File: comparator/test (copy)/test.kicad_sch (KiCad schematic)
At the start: 11 parts, among them Q4 NPN, Q5 NPN

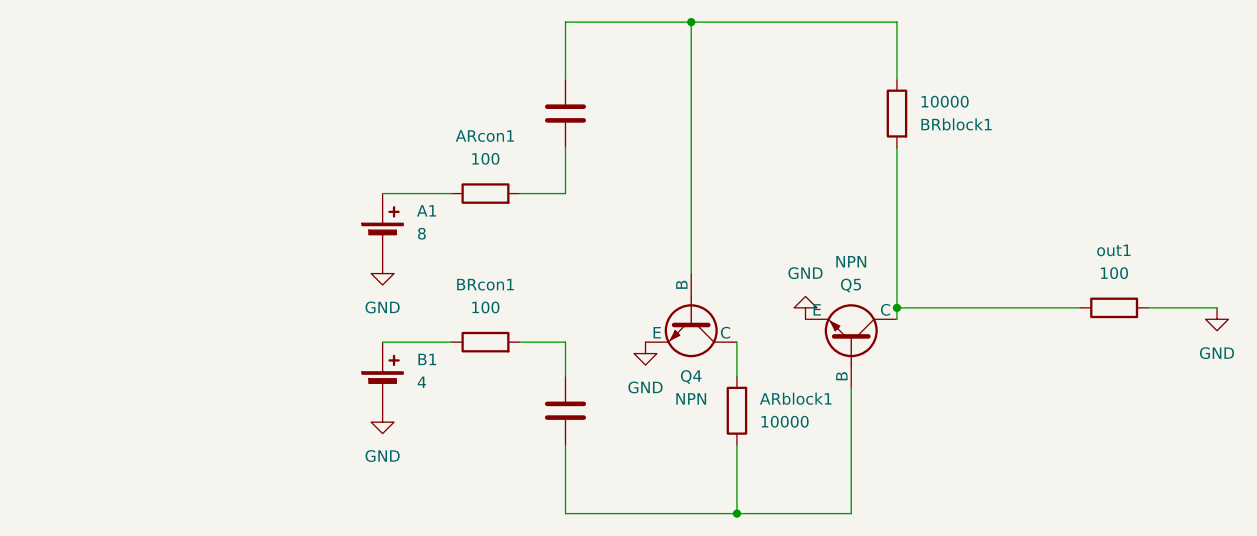
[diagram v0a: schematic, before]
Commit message: add
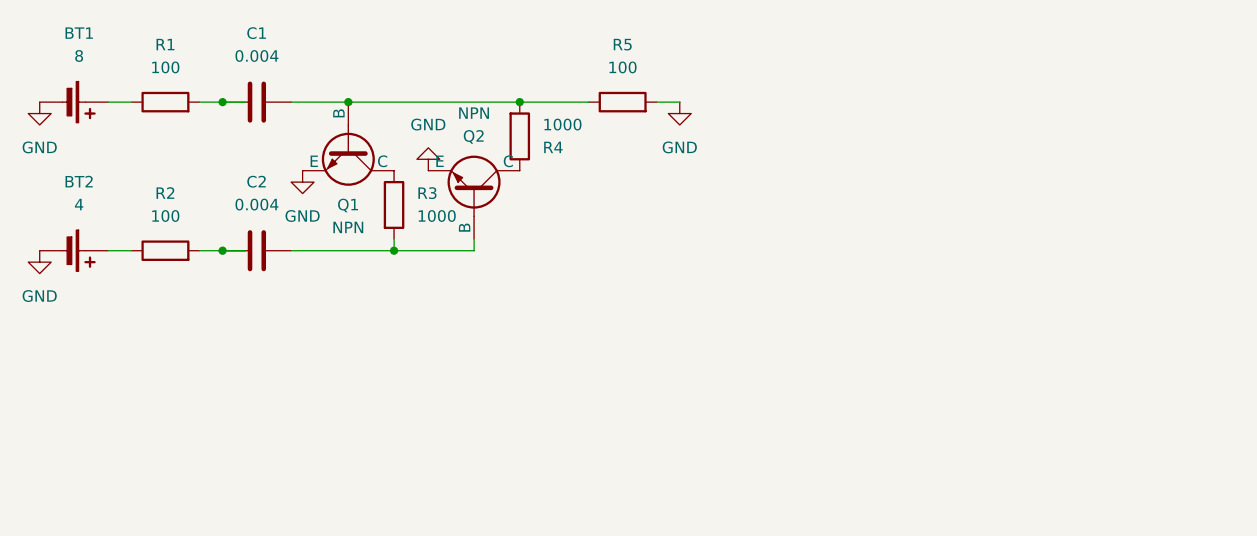
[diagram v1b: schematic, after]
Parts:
- removed A1: 8, symbol Device:Battery_Cell
- removed ARblock1, BRblock1: 10000, symbol Device:R
- removed ARcon1, BRcon1, out1: 100, symbol Device:R
- removed B1: 4, symbol Device:Battery_Cell
- removed C6, C7: 300, symbol Device:C
- removed Q4, Q5: NPN, symbol Simulation_SPICE:NPN
- added BT1: 8, symbol Device:Battery_Cell
- added BT2: 4, symbol Device:Battery_Cell
- added C1, C2: 0.004, symbol Device:C
- added Q1, Q2: NPN, symbol Simulation_SPICE:NPN
- added R1, R2, R5: 100, symbol Device:R
- added R3, R4: 1000, symbol Device:R
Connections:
- net GND: now also BT1.2 (-), BT2.2 (-), Q1.3 (E), Q2.3 (E), R5.2
- new net: Q1.1 (C), R3.1
- new net: C1.2, Q1.2 (B), R4.2, R5.1
- new net: BT2.1 (+), R2.1
- new net: C2.1, R2.2
- new net: C2.2, Q2.2 (B), R3.2
- new net: BT1.1 (+), R1.1
- new net: C1.1, R1.2
- new net: Q2.1 (C), R4.1
